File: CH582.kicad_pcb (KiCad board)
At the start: 2 copper layers, 32 x 32 mm, 51 parts, among them J1 Conn_01x02, J3 USB, J4 Conn_02x04_Odd_Even, J5 Pogo Pin Socket 2.54, Q1 NPN, N.C., U2 TP4056, U4 M3406, Y1 32MHz, Y2 Crystal_Small

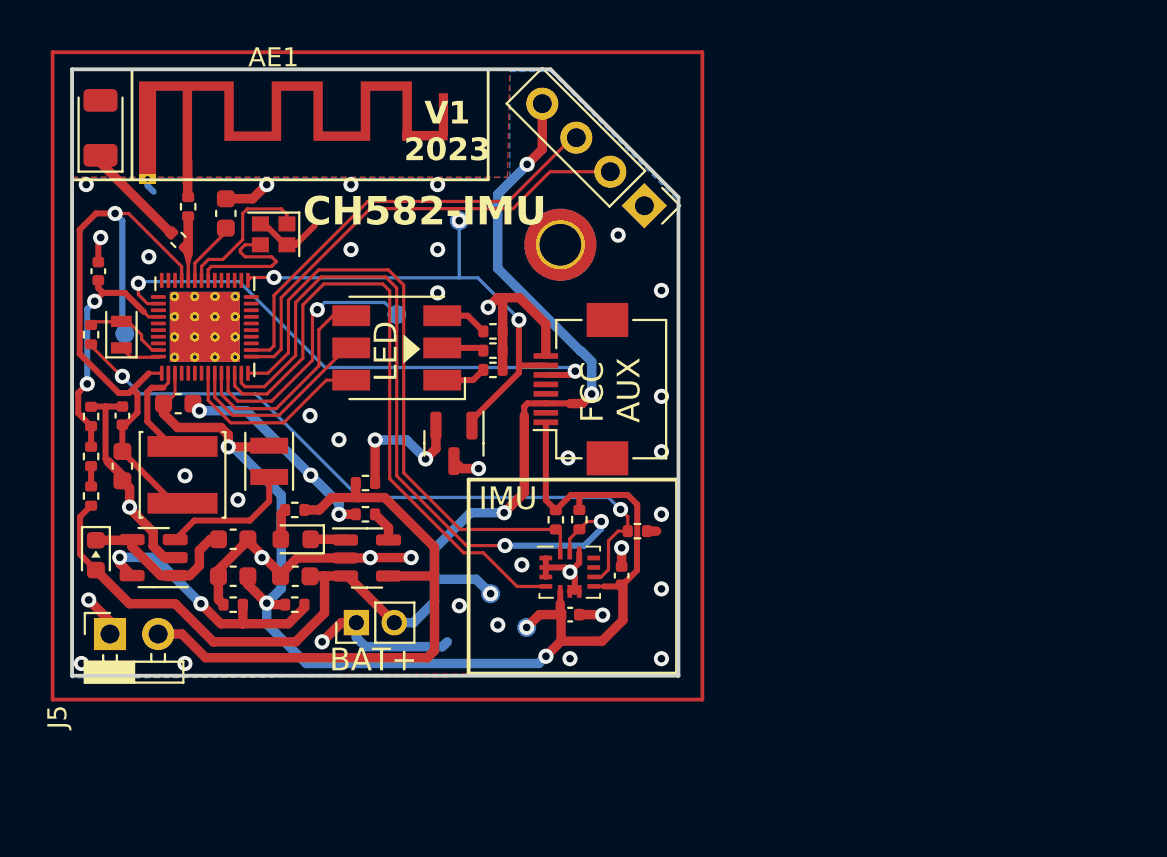
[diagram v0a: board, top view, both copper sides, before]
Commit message: V02
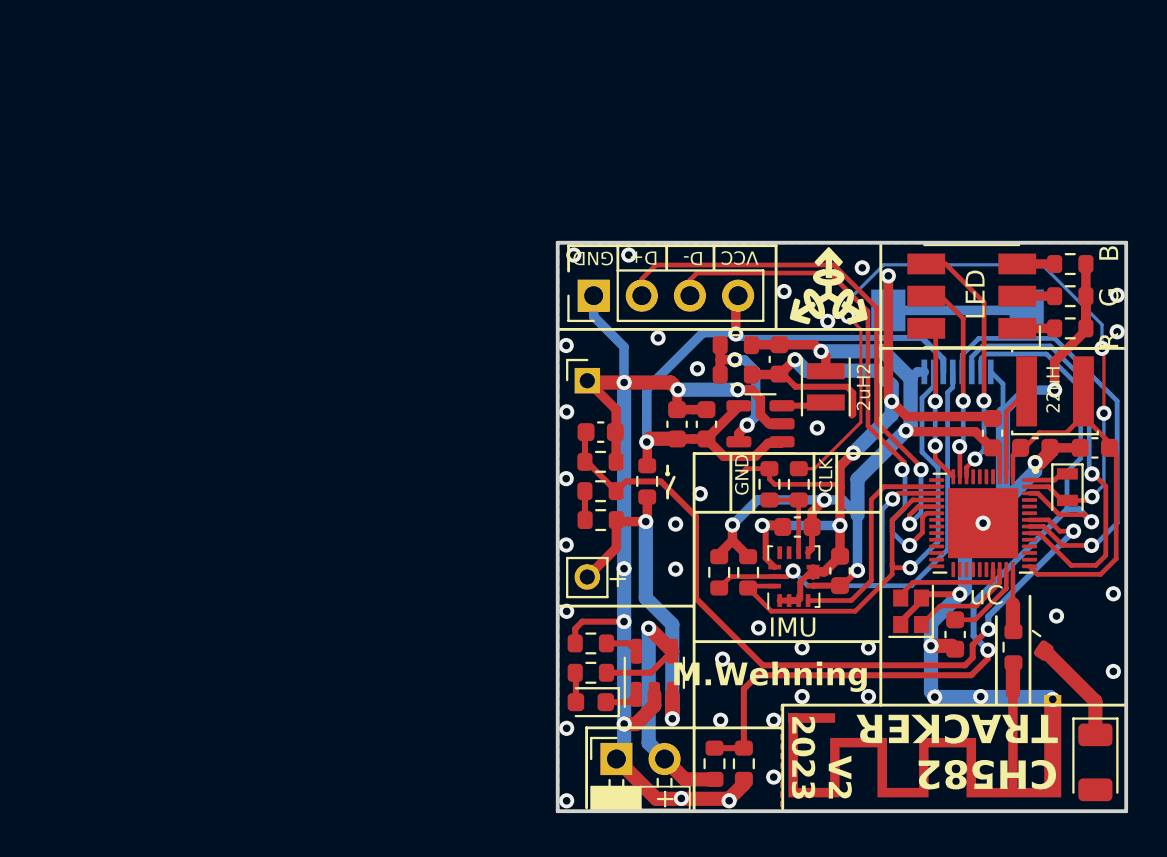
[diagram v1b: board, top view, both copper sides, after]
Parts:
- removed 3V1: 3V3, TestPoint:TestPoint_Pad_D1.0mm
- removed B+1: B+, TestPoint:TestPoint_Pad_D1.0mm
- removed D2: Schottky, Diode_SMD:D_0603_1608Metric
- removed GND1: MountingHole_Pad, MountingHole:MountingHole_2.2mm_M2_ISO14580_Pad_TopBottom
- removed Q1: NPN, N.C., Package_TO_SOT_SMD:SOT-23
- removed RST1: Reset, TestPoint:TestPoint_Pad_D1.0mm
- removed TCK1: SWD_TCK, TestPoint:TestPoint_Pad_D1.0mm
- removed VID1: VDCID, TestPoint:TestPoint_Pad_D1.0mm
- added R18: 0, Resistor_SMD:R_0603_1608Metric, F.Cu at (45.4, 36.7)
- added R19: 20k, Resistor_SMD:R_0603_1608Metric, F.Cu at (50.5, 51.6)
- C10, C2, C3, C4: footprint Capacitor_SMD:C_0402_1005Metric -> Capacitor_SMD:C_0603_1608Metric
- J4: moved to B.Cu
- J5: footprint Connector_PinSocket_2.54mm:PinSocket_1x02_P2.54mm_Horizontal -> Library:PinSocket_1x02_P2.54mm_Horizontal
- R1: value N.C. -> 10k; footprint Resistor_SMD:R_0402_1005Metric -> Resistor_SMD:R_0603_1608Metric
- R10, R11, R14, R15, R16, R17, R2, R3, R4, R5, R6, R7, R8, R9: footprint Resistor_SMD:R_0402_1005Metric -> Resistor_SMD:R_0603_1608Metric
- R12: value 316k -> 180k; footprint Resistor_SMD:R_0402_1005Metric -> Resistor_SMD:R_0603_1608Metric
- R13: value 634k -> 810k; footprint Resistor_SMD:R_0402_1005Metric -> Resistor_SMD:R_0603_1608Metric
- U2: value TP4056 -> PJ4054B
- U3: footprint Package_DFN_QFN:QFN-48-1EP_5x5mm_P0.35mm_EP3.7x3.7mm_ThermalVias -> Library:QFN 48 fixed
- moved AE2 62.3 mm to (69.0, 51.6), turned to -90 degrees
- moved AE1 51.5 mm to (64.7, 48.3), turned to 180 degrees
- moved C2 51.4 mm to (69.0, 35.0), turned to 0 degrees
- moved Y2 50.6 mm to (67.5, 37.0), turned to -90 degrees
- moved R11 49.7 mm to (65.6, 45.2), turned to -35 degrees
- moved R8 49.4 mm to (64.7, 45.5), turned to 90 degrees
- moved C8 48.2 mm to (65.8, 35.0), turned to 180 degrees
- moved L1 46.3 mm to (66.9, 32.0), turned to 0 degrees
- moved C1 44.4 mm to (61.6, 44.8), turned to 90 degrees
- moved C7 43.0 mm to (63.6, 34.2), turned to -90 degrees
- moved U3 42.4 mm to (63.1, 39.0), turned to 180 degrees
- moved Y1 39.1 mm to (59.3, 43.6), turned to 90 degrees
- moved R10 38.2 mm to (53.4, 36.9)
- moved U4 32.8 mm to (51.3, 33.7)
- moved C9 31.0 mm to (52.3, 30.3), turned to 90 degrees
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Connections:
- C5 pad 2: /B+ -> /DBG+
- C6 pad 2: Net-(D2-K) -> /DBG+
- J3 pad 4: /B+ -> /DBG+
- J4 pad 2: SDA2 -> SDA
- J4 pad 3: /B+ -> /DBG+
- J4 pad 4: SCL2 -> SCL
- R1 pad 1: Net-(Q1-B) -> G_RST
- U3 pad 10: Net-(D3-BA) -> Net-(D3-RA)
- U3 pad 25: G_RST -> unconnected-(U3-RST/TMRO_/TXD2-Pad25)
- U3 pad 41: unconnected-(U3-PA2/TMR3_-Pad41) -> INT2/DCA2
- U3 pad 46: unconnected-(U3-PA12/SCS-Pad46) -> G_RST
- U3 pad 8: Net-(D3-RA) -> Net-(D3-BA)
- U4 pad 1: Net-(D2-K) -> /DBG+
- U4 pad 4: Net-(D2-K) -> /DBG+
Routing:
- net GND: track 74.8 -> 174.3 mm, vias 41 -> 55
- net /B+: track 67.0 -> 18.8 mm, vias 4 -> 2
- net X32KO: track 4.40 -> 39.5 mm, vias 0 -> 4
- net /DBG+: track 0.00 -> 34.4 mm, vias 0 -> 2
- net ICM_CLK: track 36.6 -> 4.34 mm, vias 2 -> 0
- net ADC: track 13.2 -> 41.1 mm
- net INT2/DCA2: track 0.00 -> 22.8 mm, vias 0 -> 1
- net INT1: track 33.7 -> 11.8 mm
- net +3V3: track 66.6 -> 45.6 mm, vias 4 -> 5
- net G_RST: track 26.3 -> 47.4 mm, vias 3 -> 2
- net +5V: track 32.1 -> 16.0 mm, vias 0 -> 1
- net TCK: track 13.9 -> 0.00 mm, vias 1 -> 0
- net VDCIA: track 34.5 -> 22.0 mm, vias 1 -> 0
- net Net-(D2-K): track 8.77 -> 0.00 mm
- net SCL: track 38.8 -> 31.1 mm
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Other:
- board size 32 x 32 mm -> 30 x 30 mm
- board text added: "+"
- board text added: "22uH"
- board text added: "2uH2"
- board text added: "CH582 TRACKER"
- board text added: "CLK"
- board text added: "D+"
- board text added: "D-"
- board text added: "FCC-AUX"
- board text added: "GND"
- board text added: "M.Wehning"
- board text added: "R G B"
- board text added: "V2 2023"
- board text added: "VCC"
- board text added: "uC"
- board text removed: "BAT+"
- board text removed: "CH582-IMU"
- board text removed: "FCC AUX"
- board text removed: "V1 2023"
